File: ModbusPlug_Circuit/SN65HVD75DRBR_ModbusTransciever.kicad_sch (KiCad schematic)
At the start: 6 parts, among them U3 SN65HVD75DRBR

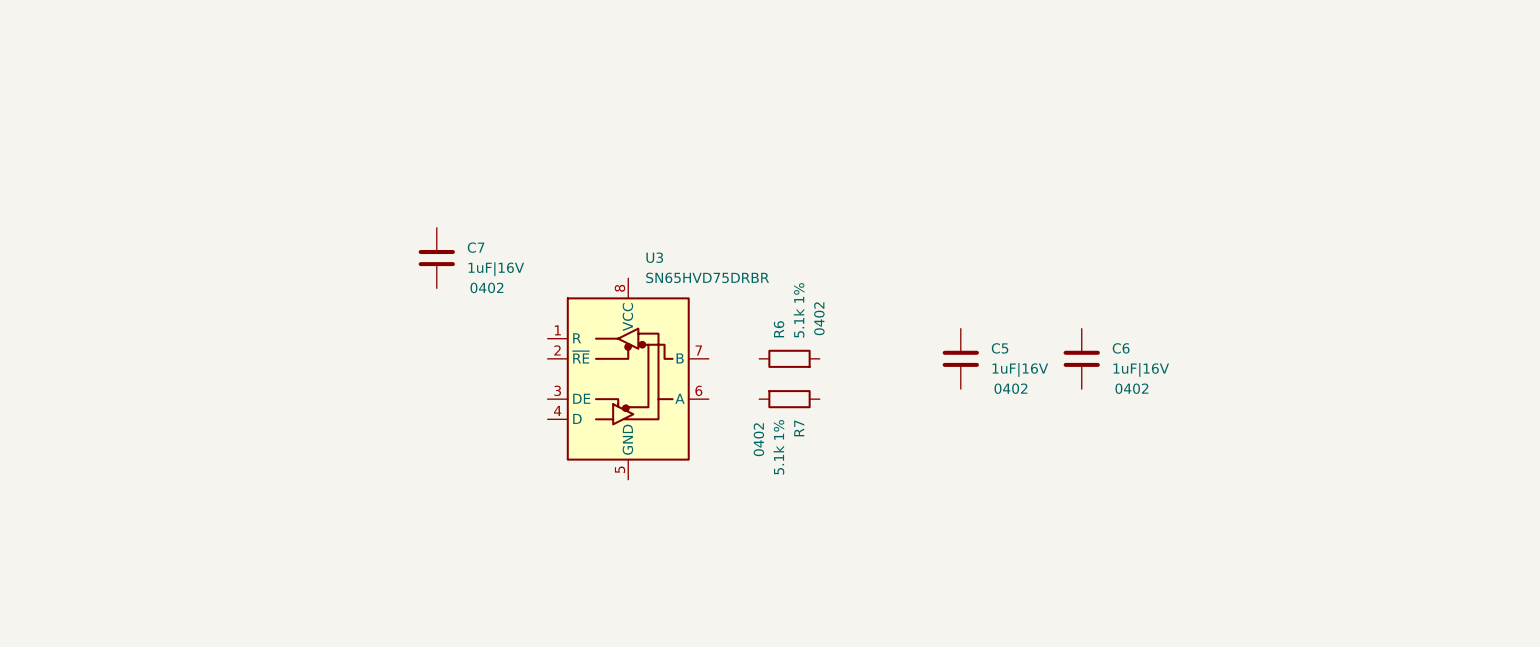
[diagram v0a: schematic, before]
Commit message: pushing V0.1
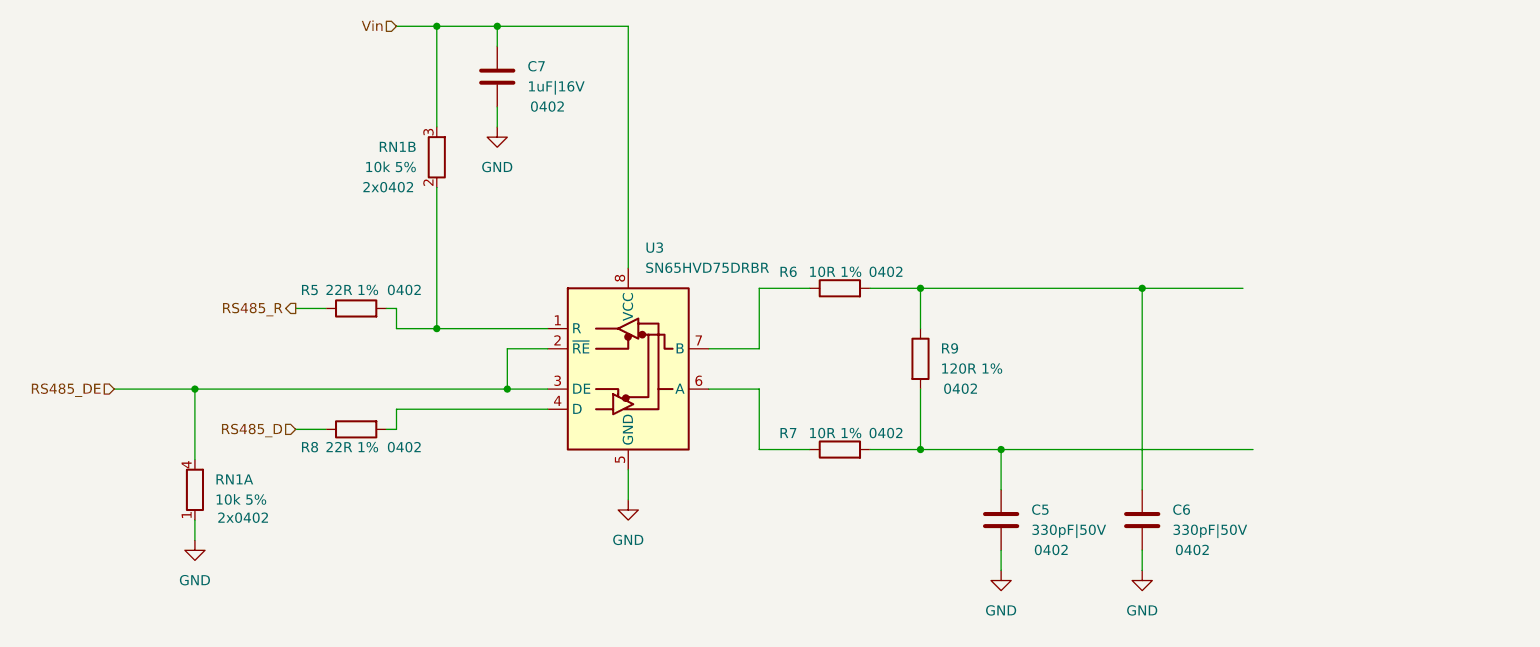
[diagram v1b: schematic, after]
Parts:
- added R5, R8: 22R 1%, Resistor_SMD:R_0402_1005Metric, symbol Device:R
- added R9: 120R 1%, Resistor_SMD:R_0402_1005Metric, symbol Device:R
- added RN1: 10k 5%, Resistor_SMD:R_Array_Convex_2x0402, symbol Device:R_Pack02_Split
- C5, C6: value 1uF|16V -> 330pF|50V
- R6, R7: value 5.1k 1% -> 10R 1%
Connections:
- net at C6.1: now also R6.2, R9.1
- net EPad: now reaches C6.2
- net EPad: now also C5.2, C7.2, U3.5 (GND), U3.9 (EPad), RN1.1 (R1.1)
- net at R7.1: now also U3.6 (A)
- net at R7.2: now also C5.1, R9.2
- net at U3.1 (R): now also R5.2, RN1.2 (R2.1)
- net RS485_DE: now reaches U3.2 (~{RE})
- net RS485_DE: now also U3.3 (DE), RN1.4 (R1.2)
- net at U3.4 (D): now also R8.2
- net at U3.7 (B): now also R6.1
- net Vin: now reaches U3.8 (VCC)
- net Vin: now also C7.1, RN1.3 (R2.2)
- new net RS485_D: R8.1
- new net RS485_R: R5.1
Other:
- moved on the sheet: C5, C6, C7, R6, U3

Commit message: pushing V0.1.1
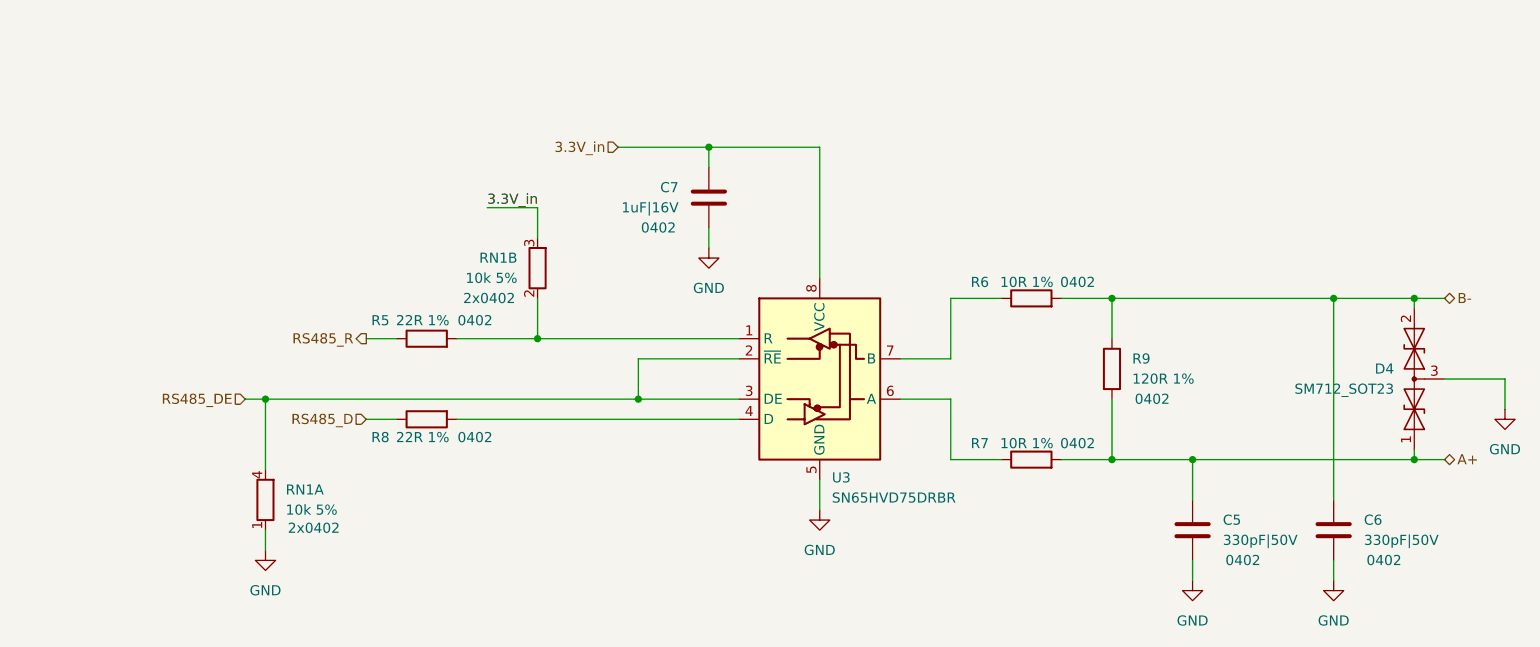
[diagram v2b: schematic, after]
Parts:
- added D4: SM712_SOT23, Package_TO_SOT_SMD:SOT-23, symbol Diode:SM712_SOT23
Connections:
- net EPad: now also D4.3 (common)
- net B-: now reaches C6.1, R6.2, R9.1
- net B-: now also D4.2 (A2)
- net A+: now reaches C5.1, R7.2, R9.2
- net A+: now also D4.1 (A1)
- net Vin renamed 3.3V_in
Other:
- moved on the sheet: C5, C6, C7, R5, R6, R7, R8, R9, RN1A, RN1B, U3
